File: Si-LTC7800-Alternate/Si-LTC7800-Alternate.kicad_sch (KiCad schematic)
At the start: 40 parts, among them Q1 BSC100N06LS3_G, Q2 BSC100N06LS3_G, U1 LTC7800HUDC_PBF

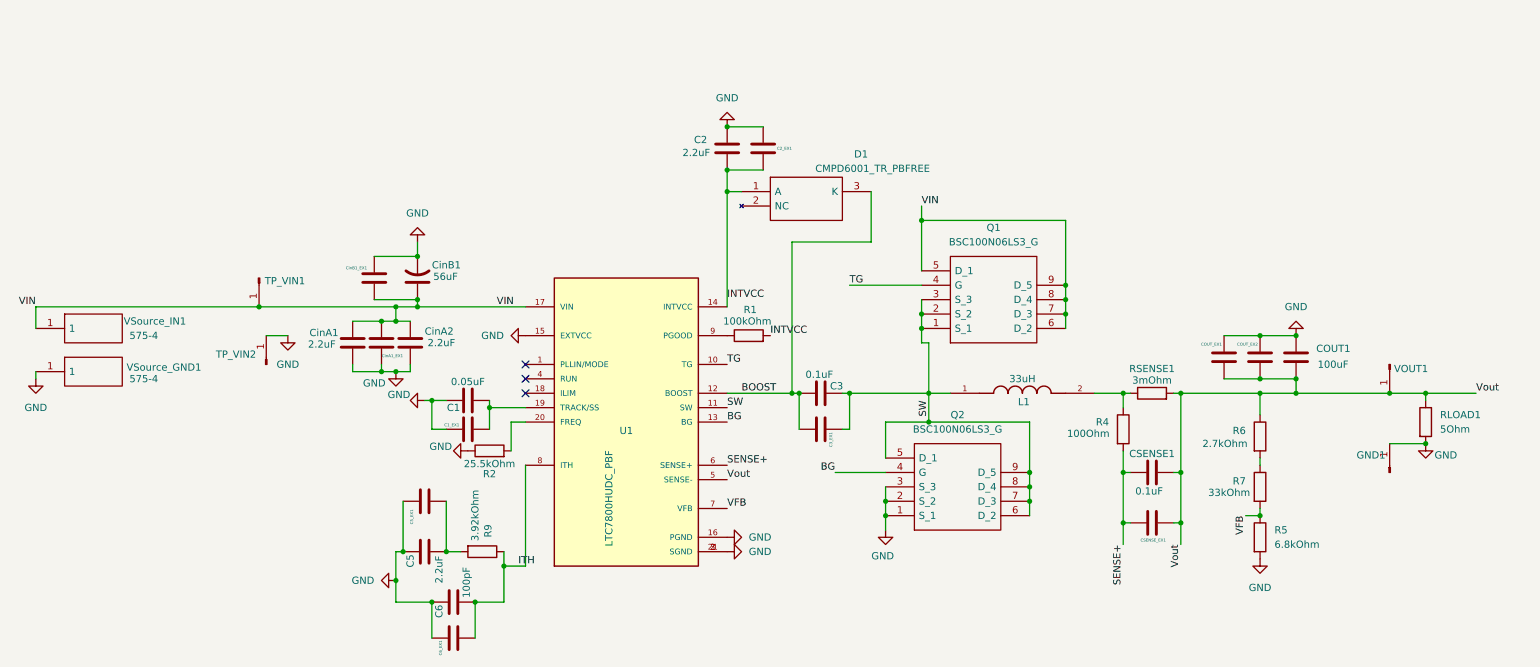
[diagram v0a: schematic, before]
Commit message: Updating PCBs for preassembly
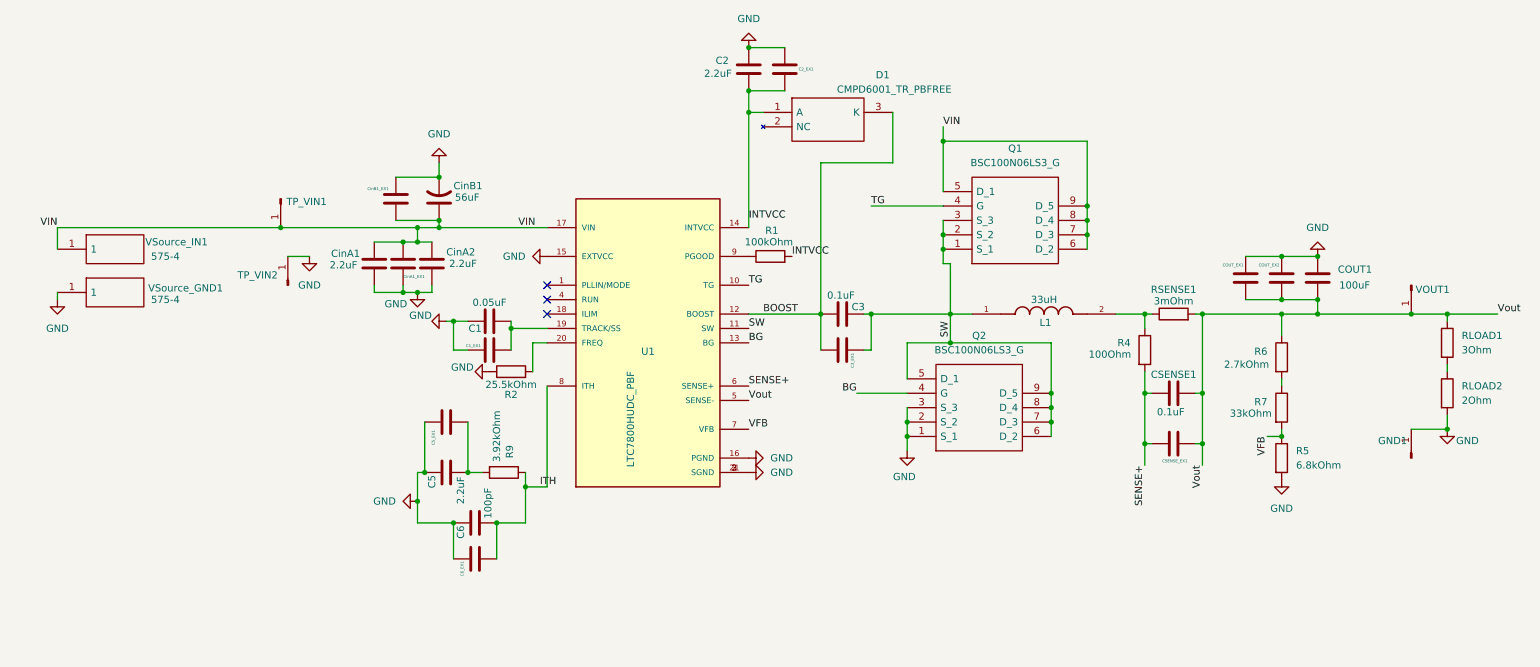
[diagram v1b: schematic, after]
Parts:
- added RLOAD2: 2Ohm, Resistor_SMD:R_0201_0603Metric, symbol Device:R
- C1, C3, CSENSE1: footprint Capacitor_SMD:C_0805_2012Metric_Pad1.18x1.45mm_HandSolder -> Capacitor_SMD:C_0805_2012Metric; LCSC (none) -> C49678
- C2, C5, CinA1, CinA2: footprint Capacitor_SMD:C_0805_2012Metric_Pad1.18x1.45mm_HandSolder -> Capacitor_SMD:C_0805_2012Metric; LCSC (none) -> C19110
- C6: footprint Capacitor_SMD:C_0805_2012Metric_Pad1.18x1.45mm_HandSolder -> Capacitor_SMD:C_0805_2012Metric; LCSC (none) -> C1970
- COUT1: footprint Capacitor_SMD:C_0805_2012Metric_Pad1.18x1.45mm_HandSolder -> Capacitor_SMD:C_0805_2012Metric; LCSC (none) -> C141660
- CinB1: footprint Capacitor_SMD:C_0805_2012Metric_Pad1.18x1.45mm_HandSolder -> Capacitor_Tantalum_SMD:CP_EIA-7343-31_Kemet-D; LCSC (none) -> C465937
- D1: LCSC (none) -> C17357273
- Q1, Q2: LCSC (none) -> C72767
- R1: footprint Resistor_SMD:R_0201_0603Metric_Pad0.64x0.40mm_HandSolder -> Resistor_SMD:R_0201_0603Metric; LCSC (none) -> C14675
- R2: footprint Resistor_SMD:R_0201_0603Metric_Pad0.64x0.40mm_HandSolder -> Resistor_SMD:R_0201_0603Metric; LCSC (none) -> C861257
- R4: footprint Resistor_SMD:R_0201_0603Metric_Pad0.64x0.40mm_HandSolder -> Resistor_SMD:R_0201_0603Metric; LCSC (none) -> C105588
- R5: footprint Resistor_SMD:R_0201_0603Metric_Pad0.64x0.40mm_HandSolder -> Resistor_SMD:R_0201_0603Metric; LCSC (none) -> C2907055
- R6: footprint Resistor_SMD:R_0201_0603Metric_Pad0.64x0.40mm_HandSolder -> Resistor_SMD:R_0201_0603Metric; LCSC (none) -> C2907008
- R7: footprint Resistor_SMD:R_0201_0603Metric_Pad0.64x0.40mm_HandSolder -> Resistor_SMD:R_0201_0603Metric; LCSC (none) -> C2907028
- R9: footprint Resistor_SMD:R_0201_0603Metric_Pad0.64x0.40mm_HandSolder -> Resistor_SMD:R_0201_0603Metric; LCSC (none) -> C4168160
- RLOAD1: value 5Ohm -> 3Ohm; footprint Resistor_SMD:R_0201_0603Metric_Pad0.64x0.40mm_HandSolder -> Resistor_SMD:R_0201_0603Metric; LCSC (none) -> C23157
- RSENSE1: footprint Resistor_SMD:R_0201_0603Metric_Pad0.64x0.40mm_HandSolder -> Resistor_SMD:R_0201_0603Metric; LCSC (none) -> C7256520
- U1: LCSC (none) -> C690192
- VSource_GND1, VSource_IN1: LCSC (none) -> C4944061
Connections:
- net GND: now also RLOAD2.2; no longer RLOAD1.2
- new net: RLOAD1.2, RLOAD2.1
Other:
- moved on the sheet: C1, C1_EX1, C2, C2_EX1, C3, C3_EX1, C5, C5_EX1, C6, C6_EX1, COUT1, COUT_EX1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
